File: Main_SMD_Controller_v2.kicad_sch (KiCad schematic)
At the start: 81 parts, among them J101 B3B-XH-A, J102 B3B-XH-A, J103 B2B-XH-A, J104 PH-1X2SG, J105 B2B-XH-A, J106 PH-1X3SG, J107 PCB-20, J108 PCB-20, J109 PCB-20, J110 PCB-20, P101 Eoshi-chan_Silk, P102 Eoshi-chan_Silk, P103 Serial_QR, U101 XC6201P332MR-G, U102 XC6902N331MR-G, U103 XC6201P502MR-G, U104 MCP1501-20E/CHY, U105 ADA4510-2ARZ, U106 NJU7098A, U107 TC4066BP, U108 LT1167CN8

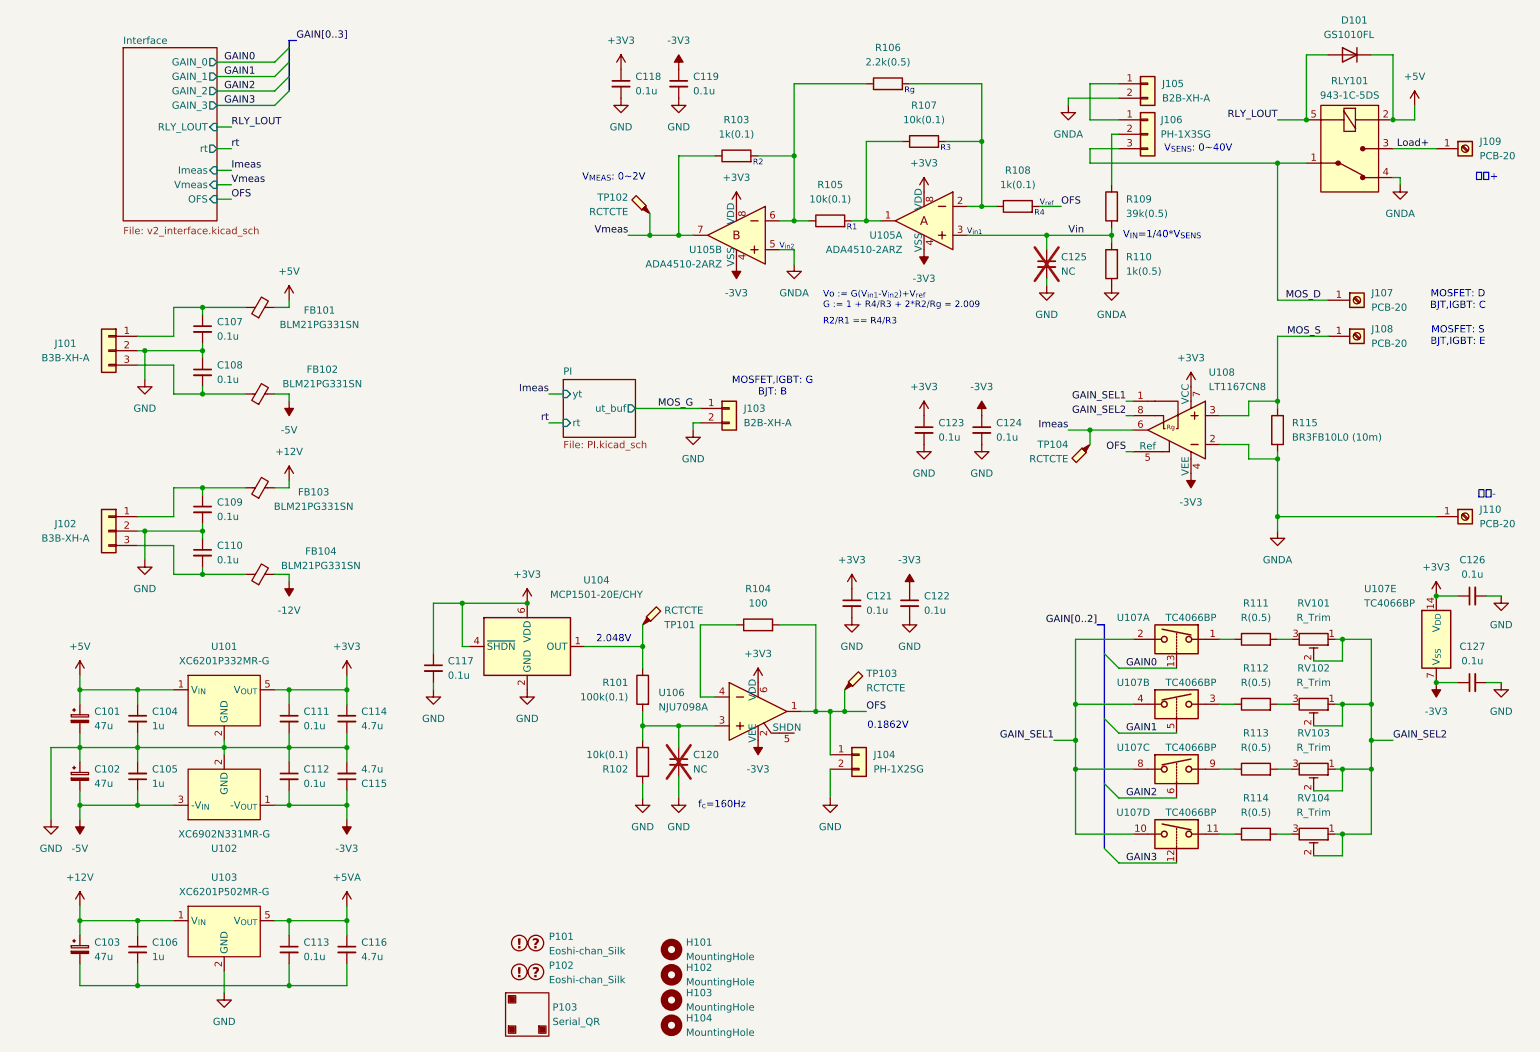
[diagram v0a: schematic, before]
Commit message: kannsei
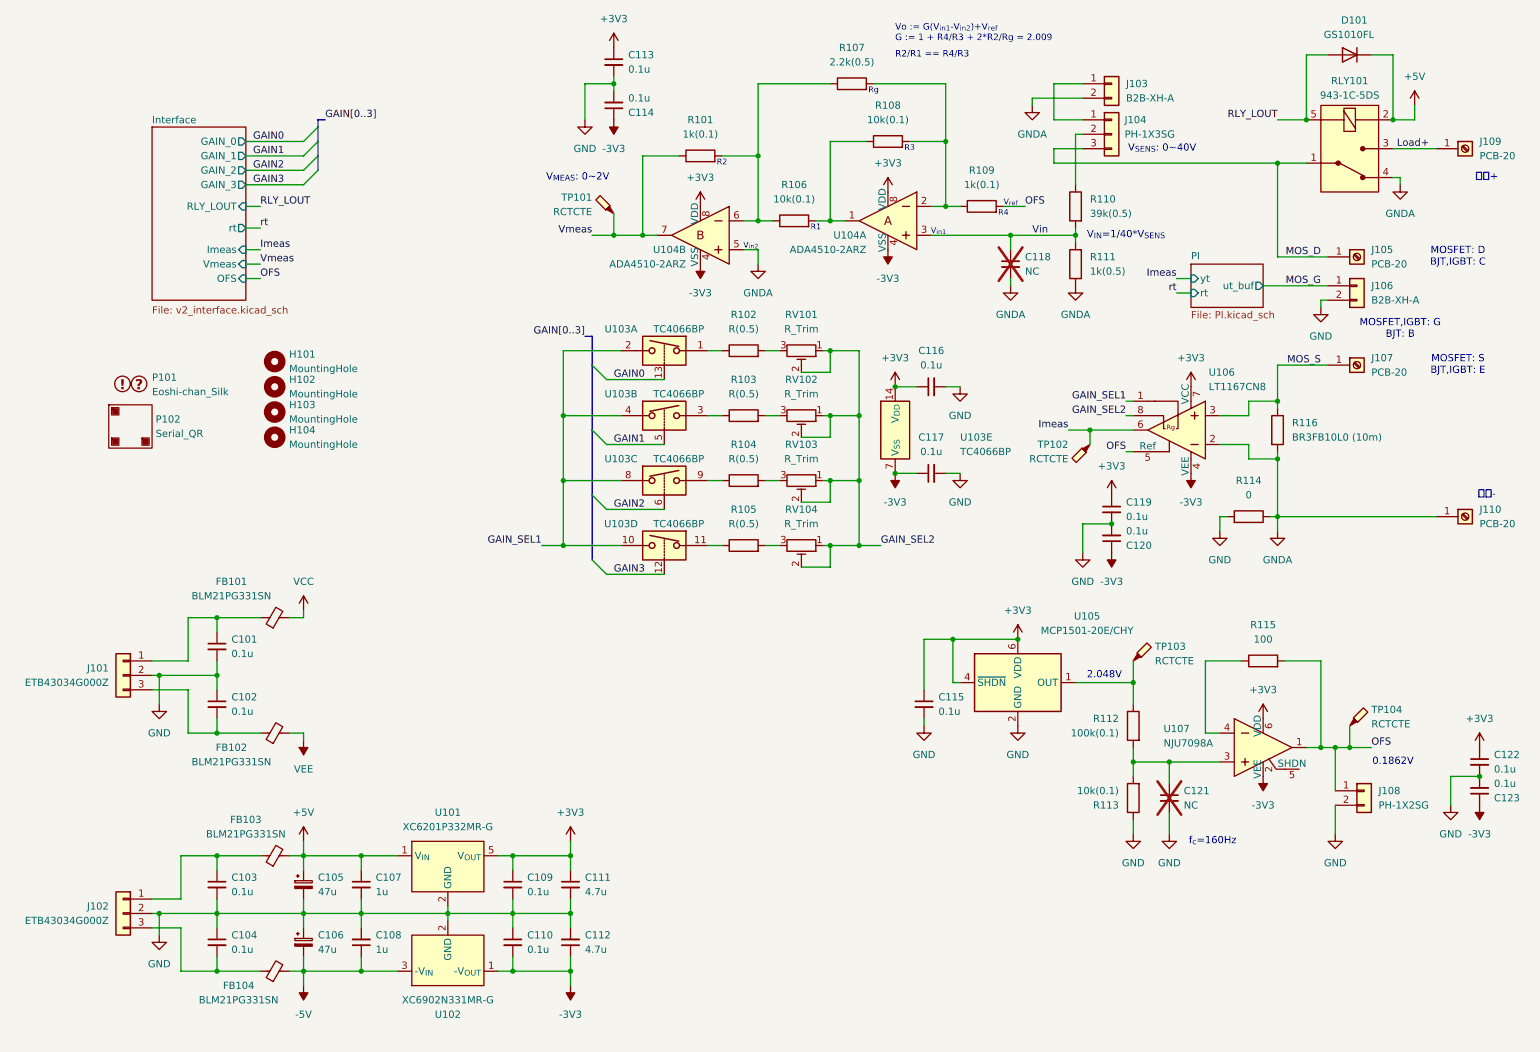
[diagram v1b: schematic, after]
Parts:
- removed C103: 47u, Capacitor_SMD:CP_Elec_6.3x5.9, symbol Device:C_Polarized_Small
- removed C106: 1u, Capacitor_SMD:C_0603_1608Metric, symbol Device:C_Small
- removed C116: 4.7u, Capacitor_SMD:C_1210_3225Metric, symbol Device:C_Small
- removed C118, C119, C121: 0.1u, Capacitor_SMD:C_0603_1608Metric, symbol Device:C_Small
- removed P101: Eoshi-chan_Silk, Eoshi-chan:Eoshi-chan_logo_15x15, symbol Eoshi-chan:Eoshi-chan_Silk
- removed U103: XC6201P502MR-G, Package_TO_SOT_SMD:SOT-23-5, symbol AM_PowerIC_Linear:XC6201P502MR-G
- added C114, C123: 0.1u, Capacitor_SMD:C_0603_1608Metric, symbol Device:C_Small
- added R114: 0, Resistor_SMD:R_0805_2012Metric, symbol Device:R
- D101: footprint Diode_THT:D_DO-41_SOD81_P10.16mm_Horizontal -> Diode_SMD:D_SOD-123F
- J101: renamed from J102; value B3B-XH-A -> ETB43034G000Z
- J102: renamed from J101; value B3B-XH-A -> ETB43034G000Z
- TP101: renamed from TP102; footprint (none) -> AM_Conn_TP:RCTCE
- TP102: renamed from TP104; footprint (none) -> AM_Conn_TP:RCTCE
- TP103: renamed from TP101; footprint (none) -> AM_Conn_TP:RCTCE
- TP104: renamed from TP103; footprint (none) -> AM_Conn_TP:RCTCE
- renumbered C109 to C101, C110 to C102, C107 to C103, C108 to C104, C101 to C105, C102 to C106, C104 to C107, C105 to C108, C111 to C109, C112 to C110, C114 to C111, C115 to C112, C117 to C115, C126 to C116, C127 to C117, C125 to C118, C123 to C119, C124 to C120, C120 to C121, FB103 to FB101, FB104 to FB102, FB101 to FB103, FB102 to FB104, J105 to J103, J106 to J104, J107 to J105, J103 to J106, J108 to J107, J104 to J108, P102 to P101, P103 to P102, R103 to R101, R111 to R102, R112 to R103, R113 to R104, R114 to R105, R105 to R106, R106 to R107, R107 to R108, R108 to R109, R109 to R110, R110 to R111, R101 to R112, R102 to R113, R104 to R115, R115 to R116, U107 to U103, U105 to U104, U104 to U105, U108 to U106, U106 to U107
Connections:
- net +5VA is gone; now on net +3V3: C113.1
- net +3V3: now also C122.1
- net -3V3: now also C114.1, C123.1; no longer C122.1
- net GND: now also C113.2, C114.2, C123.2, R114.2; no longer C118.2
- net GNDA: now also C118.2, R114.1
- net +12V renamed VCC
- net -12V renamed VEE
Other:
- company: (none) -> EosinY
- title: (none) -> Analog Controller
- moved on the sheet: C101, C102, C103, C104, C105, C106, C107, C108, C109, C110, C111, C112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
